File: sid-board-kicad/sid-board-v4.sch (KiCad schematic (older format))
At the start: 52 parts, among them J1 SPI + UART, J2 USB_B_Micro, J3 Conn_01x08, Q1 BSS138, Q2 BSS138, SW1 SW_EN, SW2 SW_FLASH, U1 SC16IS762IBS, U2 MCP1703A-3302_SOT223, U3 SN65HVD232, U4 SN65HVD232, U5 CP2102N-A01-GQFN28, U6 ESP32-WROOM-32U, U7 SN65HVD232, X1 ASE-xxxMHz

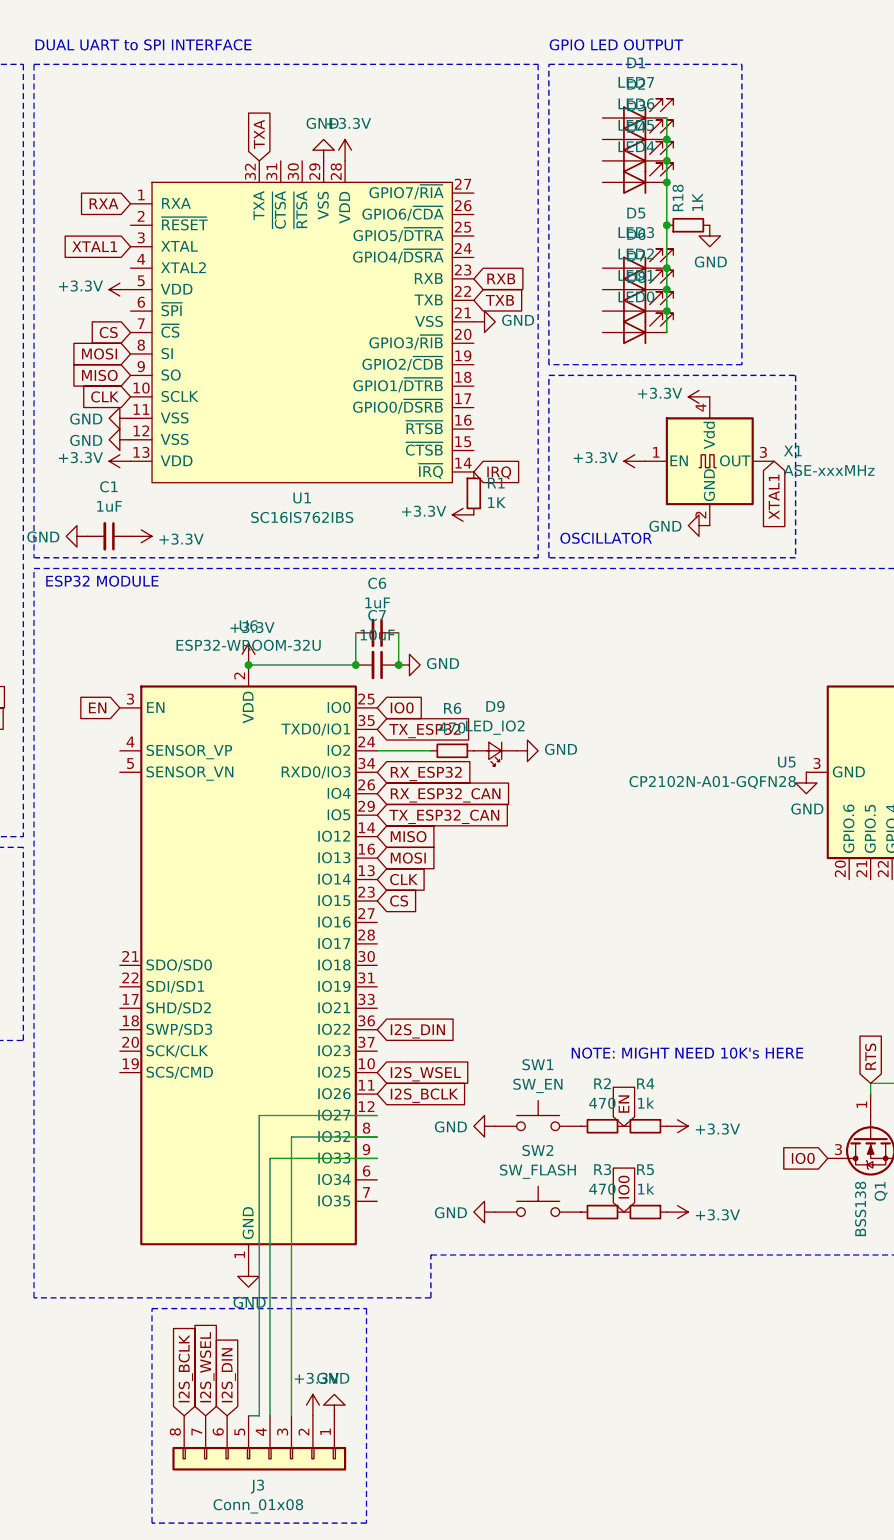
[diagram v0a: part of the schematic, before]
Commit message: Layer 4 stuff
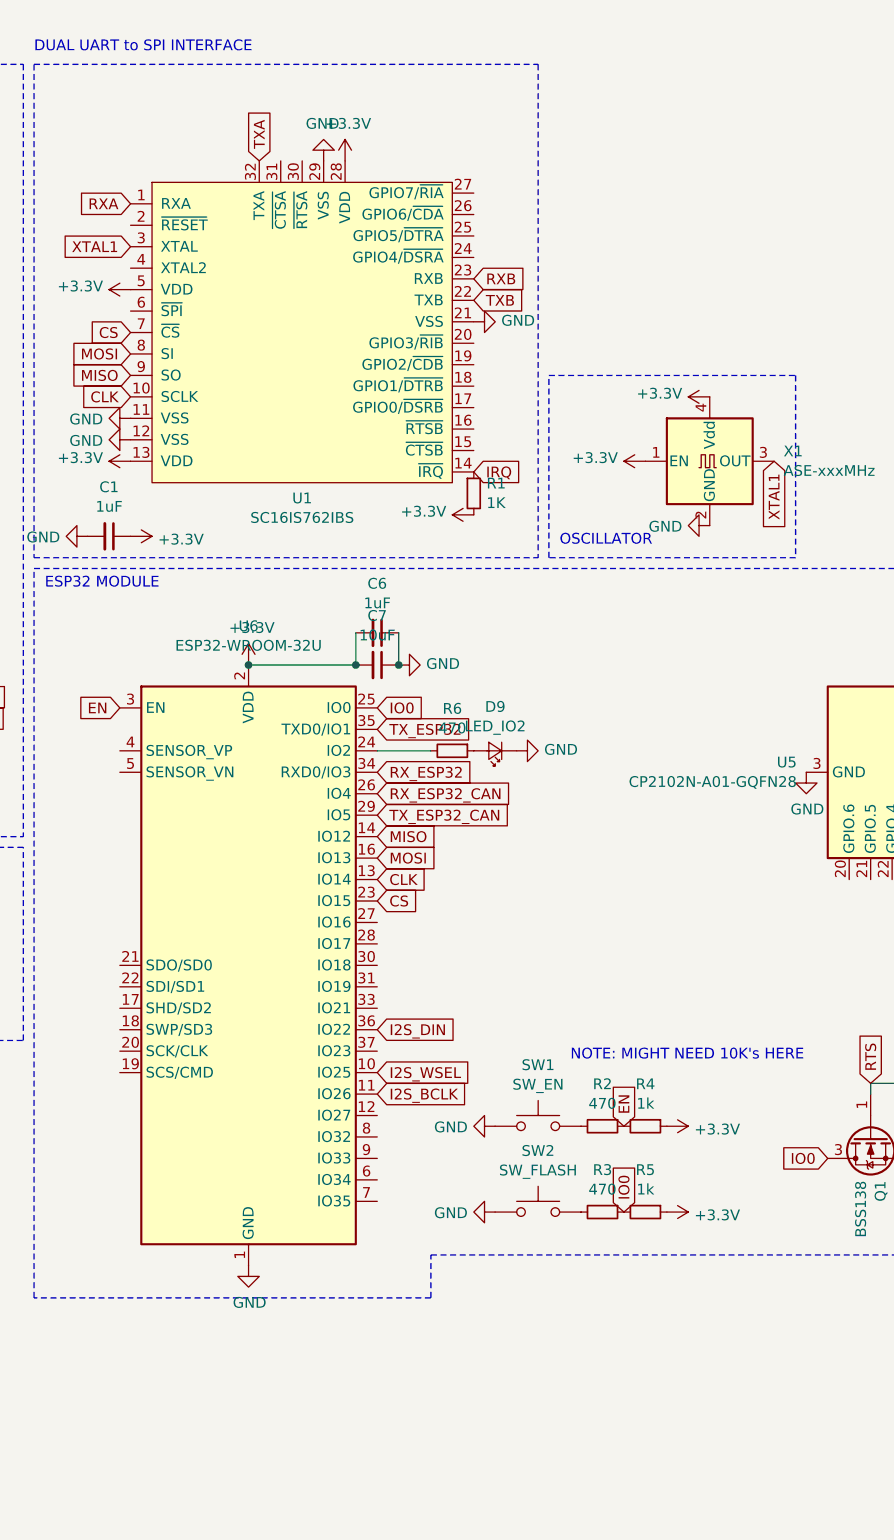
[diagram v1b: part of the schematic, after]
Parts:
- removed D1: LED7, LED_SMD:LED_0805_2012Metric_Pad1.15x1.40mm_HandSolder, symbol Device:LED
- removed D2: LED6, LED_SMD:LED_0805_2012Metric_Pad1.15x1.40mm_HandSolder, symbol Device:LED
- removed D3: LED5, LED_SMD:LED_0805_2012Metric_Pad1.15x1.40mm_HandSolder, symbol Device:LED
- removed D4: LED4, LED_SMD:LED_0805_2012Metric_Pad1.15x1.40mm_HandSolder, symbol Device:LED
- removed D5: LED3, LED_SMD:LED_0805_2012Metric_Pad1.15x1.40mm_HandSolder, symbol Device:LED
- removed D6: LED2, LED_SMD:LED_0805_2012Metric_Pad1.15x1.40mm_HandSolder, symbol Device:LED
- removed D7: LED1, LED_SMD:LED_0805_2012Metric_Pad1.15x1.40mm_HandSolder, symbol Device:LED
- removed D8: LED0, LED_SMD:LED_0805_2012Metric_Pad1.15x1.40mm_HandSolder, symbol Device:LED
- removed J3: Conn_01x08, Connector_PinHeader_2.54mm:PinHeader_1x08_P2.54mm_Vertical, symbol Connector_Generic:Conn_01x08
- removed R18: 1K, Resistor_SMD:R_0805_2012Metric_Pad1.15x1.40mm_HandSolder, symbol Device:R_Small
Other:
- note removed: "GPIO LED OUTPUT"
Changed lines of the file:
@@
 Text GLabel 7750 2700 3    50   Input ~ 0
 XTAL1
-$Comp
-L Device:LED D1
-U 1 1 5E524EBA
-P 7100 1100
-F 0 "D1" H 7093 845 50  0000 C CNN
-F 1 "LED7" H 7093 936 50  0000 C CNN
-F 2 "LED_SMD:LED_0805_2012Metric_Pad1.15x1.40mm_HandSolder" H 7100 1100 50  0001 C CNN
-F 3 "~" H 7100 1100 50  0001 C CNN
-	1    7100 1100
-	-1   0    0    1
-$EndComp
-$Comp
-L Device:LED D2
-U 1 1 5E52A67D
-P 7100 1200
-F 0 "D2" H 7093 945 50  0000 C CNN
-F 1 "LED6" H 7093 1036 50  0000 C CNN
-F 2 "LED_SMD:LED_0805_2012Metric_Pad1.15x1.40mm_HandSolder" H 7100 1200 50  0001 C CNN
-F 3 "~" H 7100 1200 50  0001 C CNN
-	1    7100 1200
-	-1   0    0    1
-$EndComp
-$Comp
-L Device:LED D3
-U 1 1 5E52A91D
-P 7100 1300
-F 0 "D3" H 7093 1045 50  0000 C CNN
-F 1 "LED5" H 7093 1136 50  0000 C CNN
-F 2 "LED_SMD:LED_0805_2012Metric_Pad1.15x1.40mm_HandSolder" H 7100 1300 50  0001 C CNN
-F 3 "~" H 7100 1300 50  0001 C CNN
-	1    7100 1300
-	-1   0    0    1
-$EndComp
-$Comp
-L Device:LED D4
-U 1 1 5E52ACF3
-P 7100 1400
-F 0 "D4" H 7093 1145 50  0000 C CNN
-F 1 "LED4" H 7093 1236 50  0000 C CNN
-F 2 "LED_SMD:LED_0805_2012Metric_Pad1.15x1.40mm_HandSolder" H 7100 1400 50  0001 C CNN
-F 3 "~" H 7100 1400 50  0001 C CNN
-	1    7100 1400
-	-1   0    0    1
-$EndComp
-$Comp
-L Device:LED D5
-U 1 1 5E52AFBB
-P 7100 1800
-F 0 "D5" H 7093 1545 50  0000 C CNN
-F 1 "LED3" H 7093 1636 50  0000 C CNN
-F 2 "LED_SMD:LED_0805_2012Metric_Pad1.15x1.40mm_HandSolder" H 7100 1800 50  0001 C CNN
-F 3 "~" H 7100 1800 50  0001 C CNN
-	1    7100 1800
-	-1   0    0    1
-$EndComp
-$Comp
-L Device:LED D6
-U 1 1 5E52B30B
-P 7100 1900
-F 0 "D6" H 7093 1645 50  0000 C CNN
-F 1 "LED2" H 7093 1736 50  0000 C CNN
-F 2 "LED_SMD:LED_0805_2012Metric_Pad1.15x1.40mm_HandSolder" H 7100 1900 50  0001 C CNN
-F 3 "~" H 7100 1900 50  0001 C CNN
-	1    7100 1900
-	-1   0    0    1
-$EndComp
-$Comp
-L Device:LED D7
-U 1 1 5E52B635
-P 7100 2000
-F 0 "D7" H 7093 1745 50  0000 C CNN
-F 1 "LED1" H 7093 1836 50  0000 C CNN
-F 2 "LED_SMD:LED_0805_2012Metric_Pad1.15x1.40mm_HandSolder" H 7100 2000 50  0001 C CNN
-F 3 "~" H 7100 2000 50  0001 C CNN
-	1    7100 2000
-	-1   0    0    1
-$EndComp
-$Comp
-L Device:LED D8
-U 1 1 5E52B939
-P 7100 2100
-F 0 "D8" H 7093 1845 50  0000 C CNN
-F 1 "LED0" H 7093 1936 50  0000 C CNN
-F 2 "LED_SMD:LED_0805_2012Metric_Pad1.15x1.40mm_HandSolder" H 7100 2100 50  0001 C CNN
-F 3 "~" H 7100 2100 50  0001 C CNN
-	1    7100 2100
-	-1   0    0    1
-$EndComp
-$Comp
-L Device:R_Small R18
-U 1 1 5E53B9FC
-P 7350 1600
-F 0 "R18" H 7409 1646 50  0000 L CNN
-F 1 "1K" H 7409 1555 50  0000 L CNN
-F 2 "Resistor_SMD:R_0805_2012Metric_Pad1.15x1.40mm_HandSolder" H 7350 1600 50  0001 C CNN
-F 3 "~" H 7350 1600 50  0001 C CNN
-	1    7350 1600
-	0    -1   -1   0
-$EndComp
-Connection ~ 7250 1200
-Wire Wire Line
-	7250 1200 7250 1100
-Connection ~ 7250 1300
-Wire Wire Line
-	7250 1300 7250 1200
-Wire Wire Line
-	7250 1400 7250 1300
-Connection ~ 7250 1900
-Wire Wire Line
-	7250 1900 7250 1800
-Connection ~ 7250 2000
-Wire Wire Line
-	7250 2000 7250 1900
-Wire Wire Line
-	7250 2100 7250 2000
-Wire Notes Line
-	6700 850  7600 850
-Wire Notes Line
-	7600 2250 6700 2250
-Wire Notes Line
-	6700 2250 6700 850
-Text Notes 6700 800  0    50   ~ 0
-GPIO LED OUTPUT
 Text GLabel 4750 2400 0    50   Input ~ 0
 CLK
@@
 Wire Notes Line
 	4250 4500 2250 4500
-Wire Wire Line
-	7250 1600 7250 1400
-Connection ~ 7250 1400
-Wire Wire Line
-	7250 1600 7250 1800
-Connection ~ 7250 1600
-Connection ~ 7250 1800
-Wire Notes Line
-	7600 850  7600 2250
 $Comp
 L Device:C_Small C6
@@
 	1    0    0    -1
 $EndComp
-$Comp
-L Connector_Generic:Conn_01x08 J3
-U 1 1 5F374BE1
-P 5400 7350
-F 0 "J3" V 5525 7296 50  0000 C CNN
-F 1 "Conn_01x08" V 5616 7296 50  0000 C CNN
-F 2 "Connector_PinHeader_2.54mm:PinHeader_1x08_P2.54mm_Vertical" H 5400 7350 50  0001 C CNN
-F 3 "~" H 5400 7350 50  0001 C CNN
-	1    5400 7350
-	0    1    1    0
-$EndComp
 Text GLabel 5900 5350 2    50   Input ~ 0
 I2S_DIN
@@
 Text GLabel 5900 5650 2    50   Input ~ 0
 I2S_BCLK
-Text GLabel 5200 7150 1    50   Input ~ 0
-I2S_DIN
-Text GLabel 5100 7150 1    50   Input ~ 0
-I2S_WSEL
-Text GLabel 5000 7150 1    50   Input ~ 0
-I2S_BCLK
-Wire Wire Line
-	5900 5950 5400 5950
-Wire Wire Line
-	5400 5950 5400 7150
-Wire Wire Line
-	5900 5850 5500 5850
-Wire Wire Line
-	5500 5850 5500 7150
-Wire Wire Line
-	5900 5750 5350 5750
-Wire Wire Line
-	5350 5750 5350 7150
-Wire Wire Line
-	5350 7150 5300 7150
-Wire Notes Line
-	4850 6650 5850 6650
-Wire Notes Line
-	5850 6650 5850 7650
-Wire Notes Line
-	5850 7650 4850 7650
-Wire Notes Line
-	4850 7650 4850 6650
 Text GLabel 10000 4650 3    50   Input ~ 0
 RX_ESP32
@@
 $EndComp
 $Comp
-L power:GND #PWR0120
-U 1 1 5F547763
-P 7450 1600
-F 0 "#PWR0120" H 7450 1350 50  0001 C CNN
-F 1 "GND" H 7455 1427 50  0000 C CNN
-F 2 "" H 7450 1600 50  0001 C CNN
-F 3 "" H 7450 1600 50  0001 C CNN
-	1    7450 1600
-	1    0    0    -1
-$EndComp
-$Comp
 L power:GND #PWR0121
 U 1 1 5F549615
@@
 Connection ~ 5300 3650
 $Comp
-L power:+3.3V #PWR0134
-U 1 1 5F572C6A
-P 5600 7150
-F 0 "#PWR0134" H 5600 7000 50  0001 C CNN
-F 1 "+3.3V" H 5615 7323 50  0000 C CNN
-F 2 "" H 5600 7150 50  0001 C CNN
-F 3 "" H 5600 7150 50  0001 C CNN
-	1    5600 7150
-	1    0    0    -1
-$EndComp
-$Comp
-L power:GND #PWR0135
-U 1 1 5F573E82
-P 5700 7150
-F 0 "#PWR0135" H 5700 6900 50  0001 C CNN
-F 1 "GND" H 5705 6977 50  0000 C CNN
-F 2 "" H 5700 7150 50  0001 C CNN
-F 3 "" H 5700 7150 50  0001 C CNN
-	1    5700 7150
-	-1   0    0    1
-$EndComp
-$Comp
 L power:+3.3V #PWR0136
